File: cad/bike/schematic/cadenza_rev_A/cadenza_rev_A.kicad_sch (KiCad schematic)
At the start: 37 parts, among them J1 USB_A, J2 USB_C_Receptacle, J3 Conn_01x02, Q1 BC547, U1 TLC5916, U10 HDSP-A151, U11 TLC5916, U12 HDSP-A151, U13 STM32F105RCTx, U14 INA193, U15 TLC5916, U2 HDSP-A151, U3 TLC5916, U4 HDSP-A151, U5 TLC5916, U6 HDSP-A151, U7 TLC5916, U8 HDSP-A151, U9 TLC5916

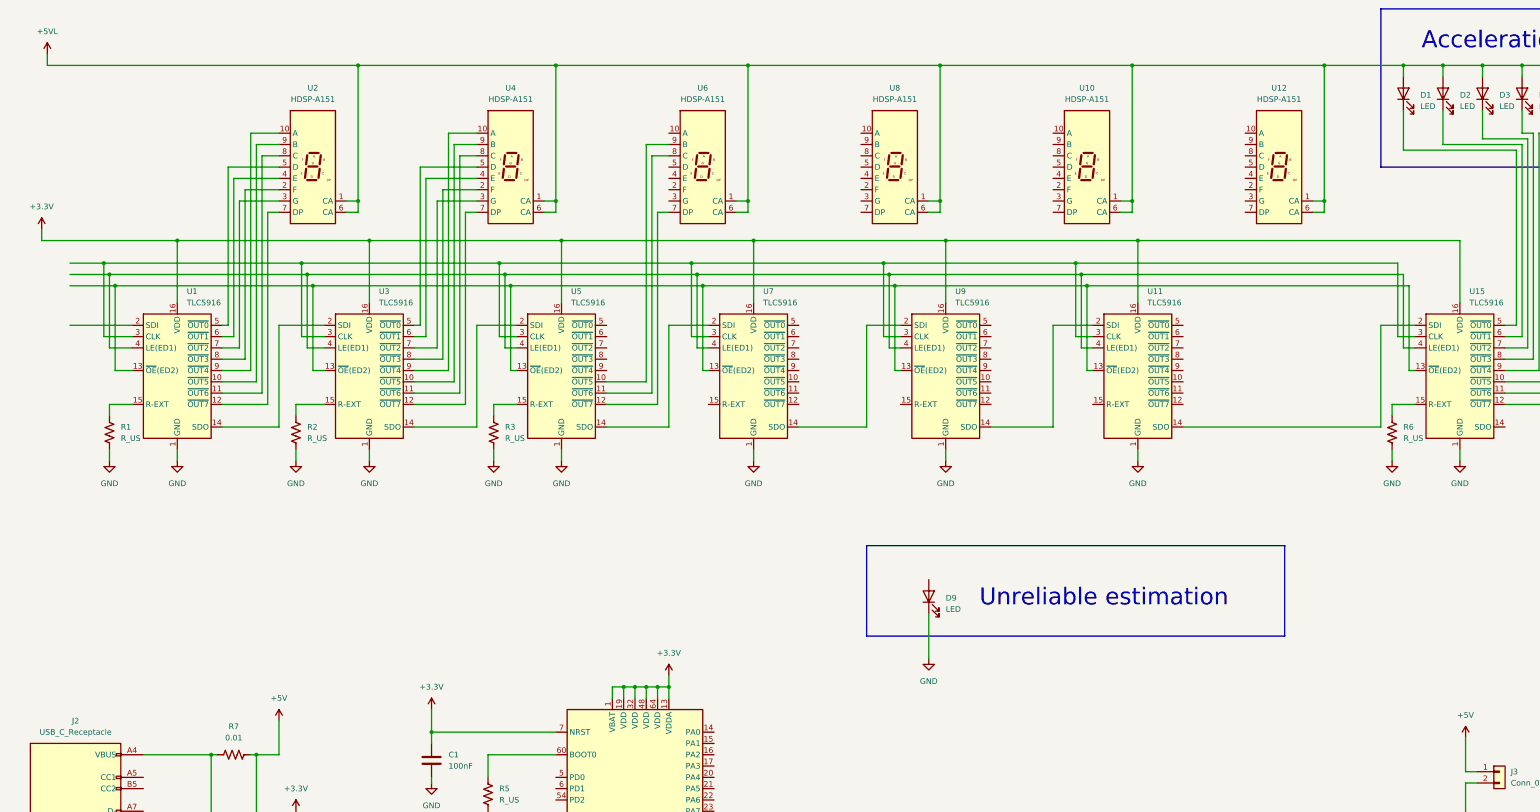
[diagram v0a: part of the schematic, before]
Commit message: routing progress update
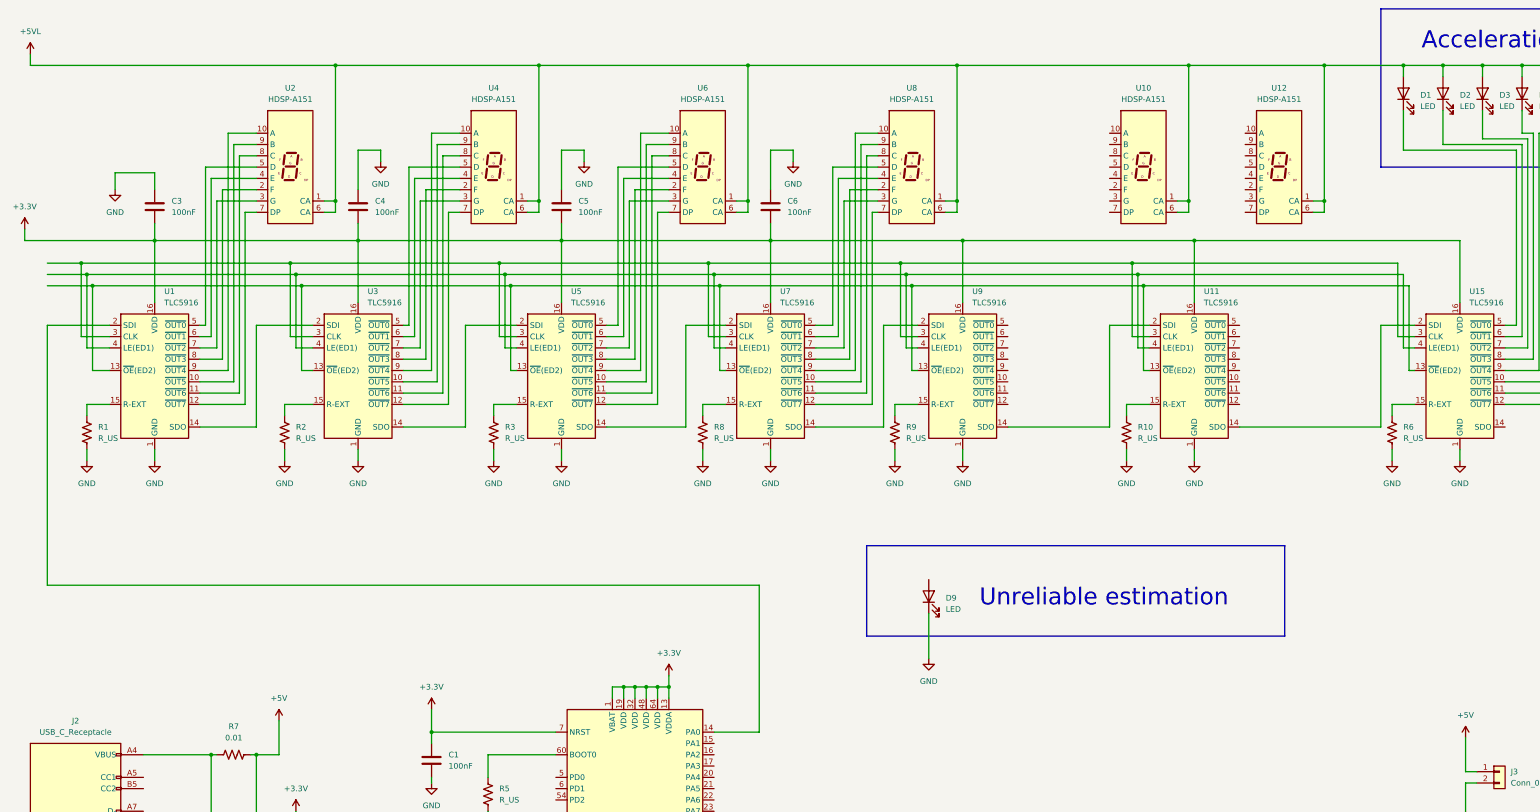
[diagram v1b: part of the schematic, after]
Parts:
- added C3, C4, C5, C6: 100nF, Capacitor_SMD:C_0805_2012Metric_Pad1.18x1.45mm_HandSolder, symbol Device:C
- added R10, R8, R9: R_US, Resistor_SMD:R_0805_2012Metric_Pad1.20x1.40mm_HandSolder, symbol Device:R_US
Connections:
- net +3.3V: now also C3.2, C4.2, C5.2, C6.2
- net GND: now also C3.1, C4.1, C5.1, C6.1, R10.2, R8.2, R9.2
- net at U9.15 (R-EXT): now also R9.1
- net at U13.14 (PA0): now also U1.2 (SDI)
- net at U7.10 (~{OUT5}): now also U8.9 (B)
- net at U7.11 (~{OUT6}): now also U8.8 (C)
- net at U7.12 (~{OUT7}): now also U8.7 (DP)
- net at U7.15 (R-EXT): now also R8.1
- net at U7.5 (~{OUT0}): now also U8.5 (D)
- net at U7.6 (~{OUT1}): now also U8.4 (E)
- net at U7.7 (~{OUT2}): now also U8.3 (G)
- net at U7.8 (~{OUT3}): now also U8.2 (F)
- net at U7.9 (~{OUT4}): now also U8.10 (A)
- net at U11.15 (R-EXT): now also R10.1
- net at U6.10 (A): now also U5.9 (~{OUT4})
- net at U6.2 (F): now also U5.8 (~{OUT3})
- net at U6.3 (G): now also U5.7 (~{OUT2})
- net at U6.4 (E): now also U5.6 (~{OUT1})
- net at U6.5 (D): now also U5.5 (~{OUT0})
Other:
- moved on the sheet: R1, R2, U1, U10, U11, U2, U3, U4, U7, U8, U9

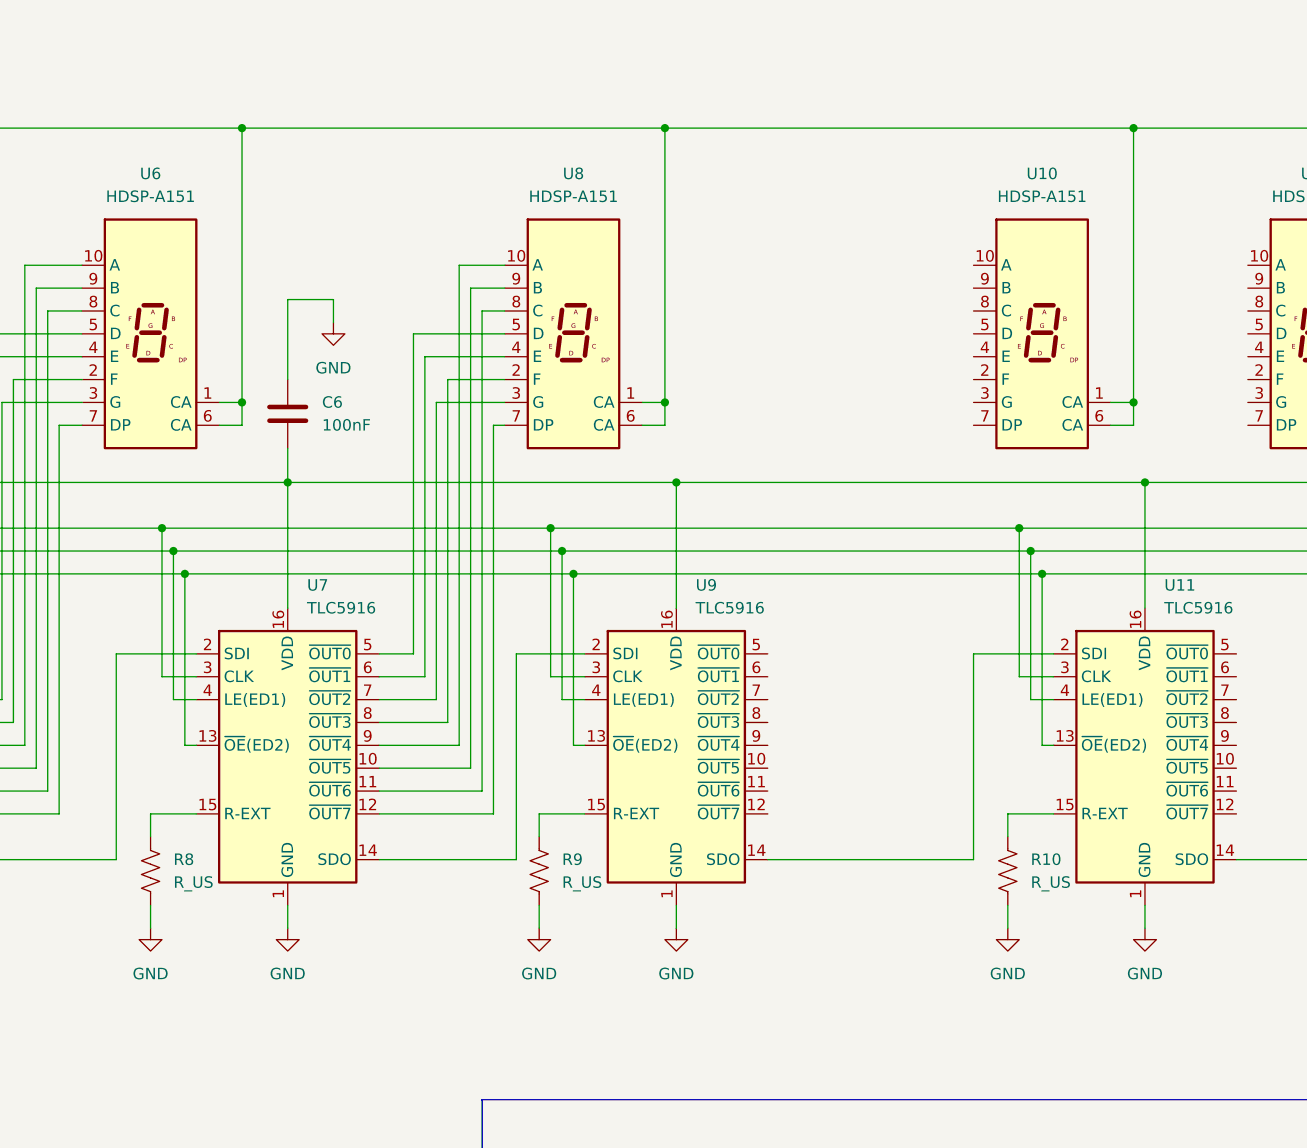
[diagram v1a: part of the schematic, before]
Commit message: switched to a new estimator
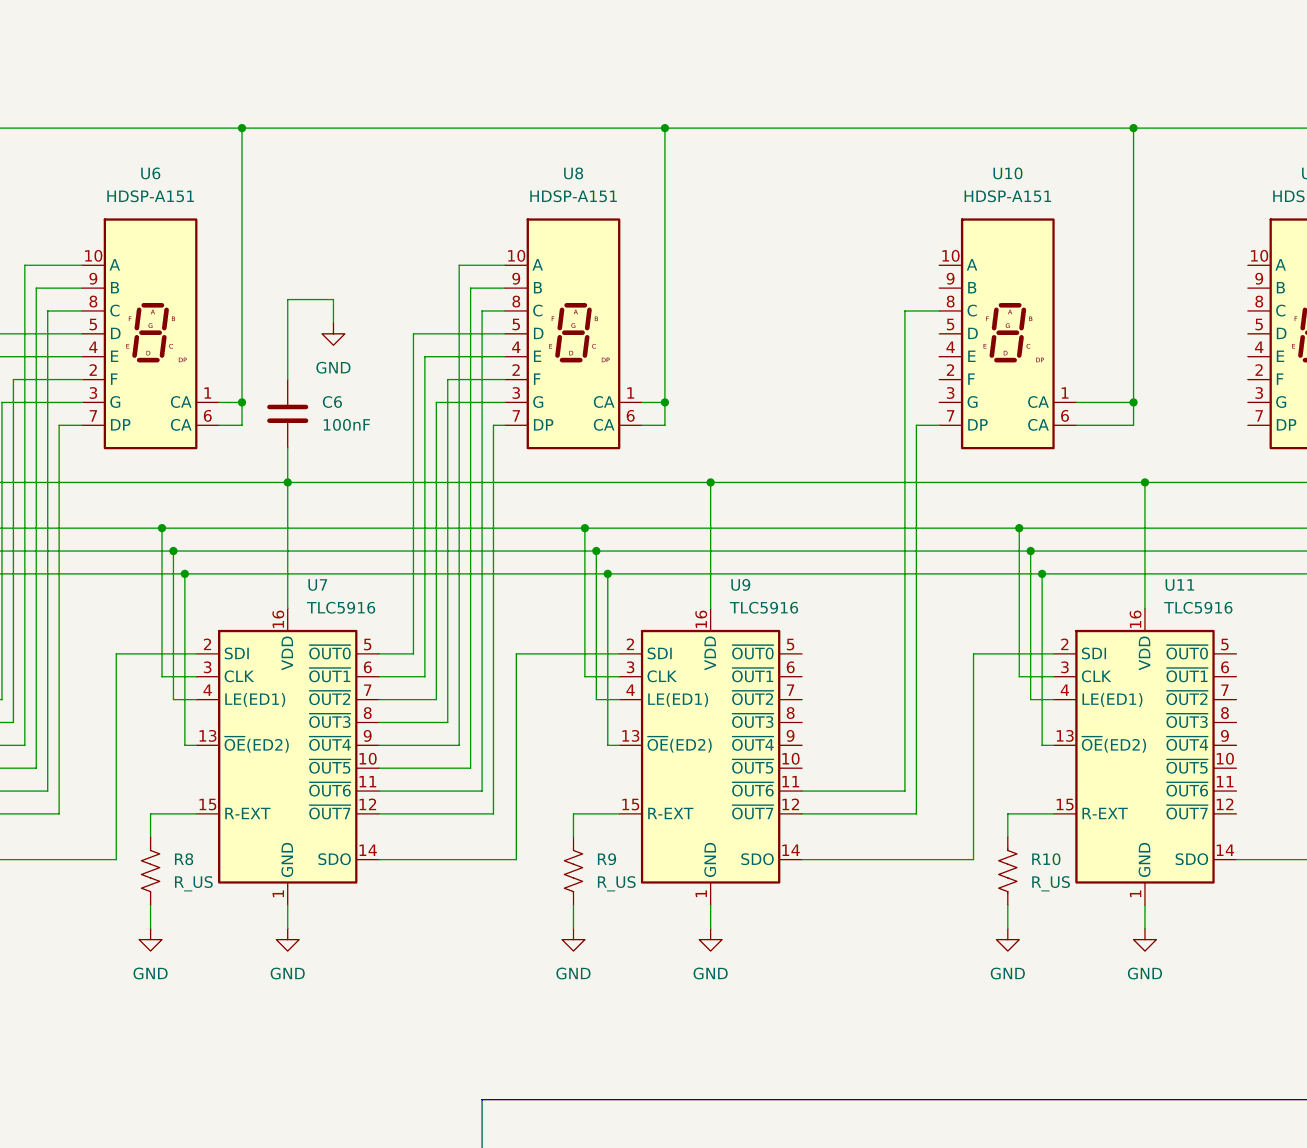
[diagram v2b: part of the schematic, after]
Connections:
- net at U9.11 (~{OUT6}): now also U10.8 (C)
- net at U9.12 (~{OUT7}): now also U10.7 (DP)
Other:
- moved on the sheet: R9, U10, U9

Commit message: routing progress update
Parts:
- added C7, C8: 100nF, Capacitor_SMD:C_0805_2012Metric_Pad1.18x1.45mm_HandSolder, symbol Device:C
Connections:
- net +3.3V: now also C7.2, C8.2
- net GND: now also C7.1, C8.1
- net at U9.10 (~{OUT5}): now also U10.9 (B)
- net at U9.5 (~{OUT0}): now also U10.5 (D)
- net at U9.6 (~{OUT1}): now also U10.4 (E)
- net at U9.7 (~{OUT2}): now also U10.3 (G)
- net at U9.8 (~{OUT3}): now also U10.2 (F)
- net at U9.9 (~{OUT4}): now also U10.10 (A)
- net at U11.10 (~{OUT5}): now also U12.9 (B)
- net at U11.11 (~{OUT6}): now also U12.8 (C)
- net at U11.12 (~{OUT7}): now also U12.7 (DP)
- net at U11.5 (~{OUT0}): now also U12.5 (D)
- net at U11.6 (~{OUT1}): now also U12.4 (E)
- net at U11.7 (~{OUT2}): now also U12.3 (G)
- net at U11.8 (~{OUT3}): now also U12.2 (F)
- net at U11.9 (~{OUT4}): now also U12.10 (A)
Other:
- moved on the sheet: C3, C4, C5, C6, D1, D2, D3, D4, D5, D6, D7, D8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
